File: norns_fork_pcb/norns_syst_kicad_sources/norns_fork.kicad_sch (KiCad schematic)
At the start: 51 parts, among them J1 ENC_K1, J10 Raspberry_Pi_2_3, J11 Ecran_SSD1306, J2 ENC_K2, J3 ENC_K3, J4 ENC_K4, J5 Conn_audio_headphone, J6 conn_headphone_up, J7 Conn_audio_INPUT, J8 conn_input_up, J9 ecran, K1 BP_K1, K2 BP_K2, K3 BP_K3

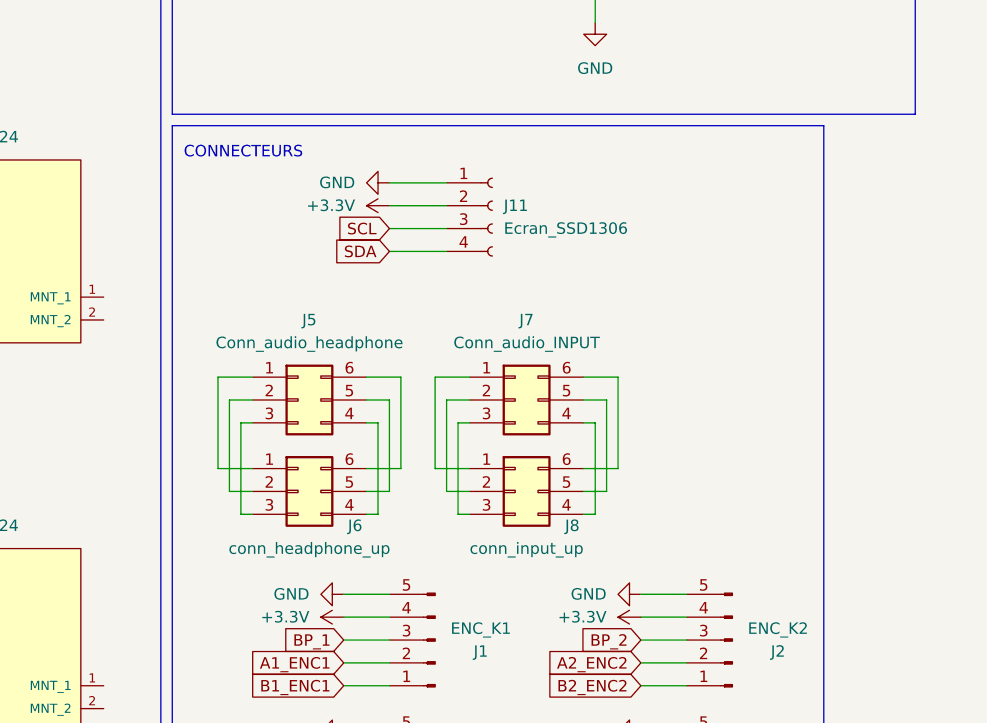
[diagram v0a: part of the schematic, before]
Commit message: mise a jour du PCB
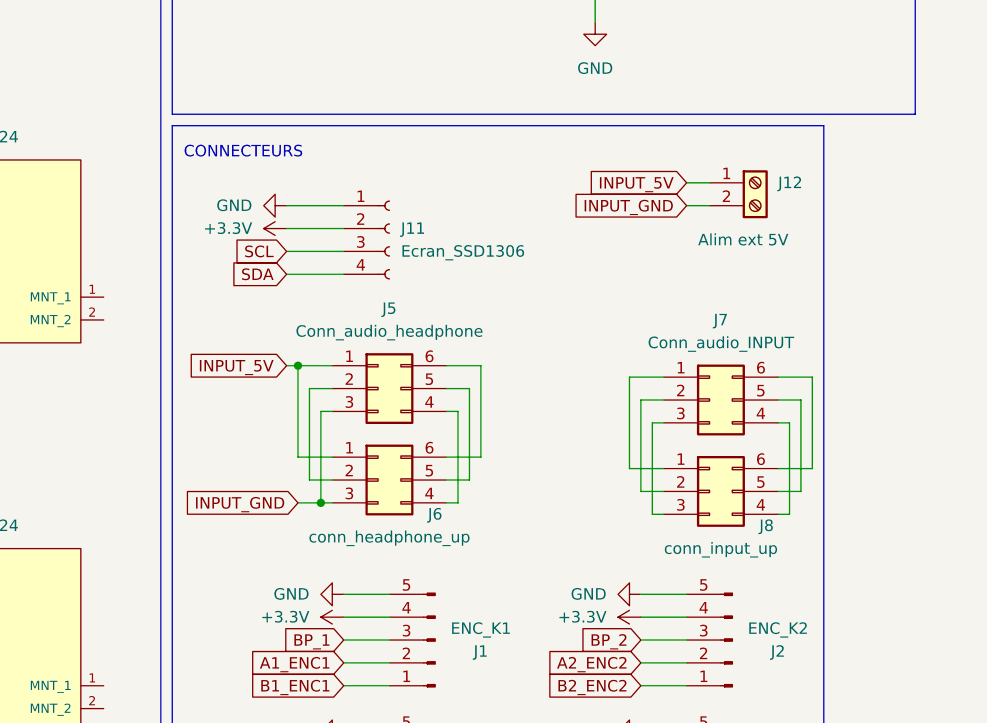
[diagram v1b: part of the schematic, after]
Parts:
- added J12: Alim ext 5V, symbol Connector:Screw_Terminal_01x02
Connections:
- net INPUT_5V: now reaches J5.1 (Pin_1), J6.1 (Pin_1)
- net INPUT_5V: now also J12.1 (Pin_1)
- net INPUT_GND: now reaches J5.3 (Pin_3), J6.3 (Pin_3)
- net INPUT_GND: now also J12.2 (Pin_2)
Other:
- moved on the sheet: J11, J5, J6, J7, J8
